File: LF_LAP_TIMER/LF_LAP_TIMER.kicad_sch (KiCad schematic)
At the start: 13 parts, among them J1 LCD I2C EXPANDER, K1 G6E, SW1 ARM, SW2 STOP, SW3 RESTART, SW4 OBJECT DETECTING

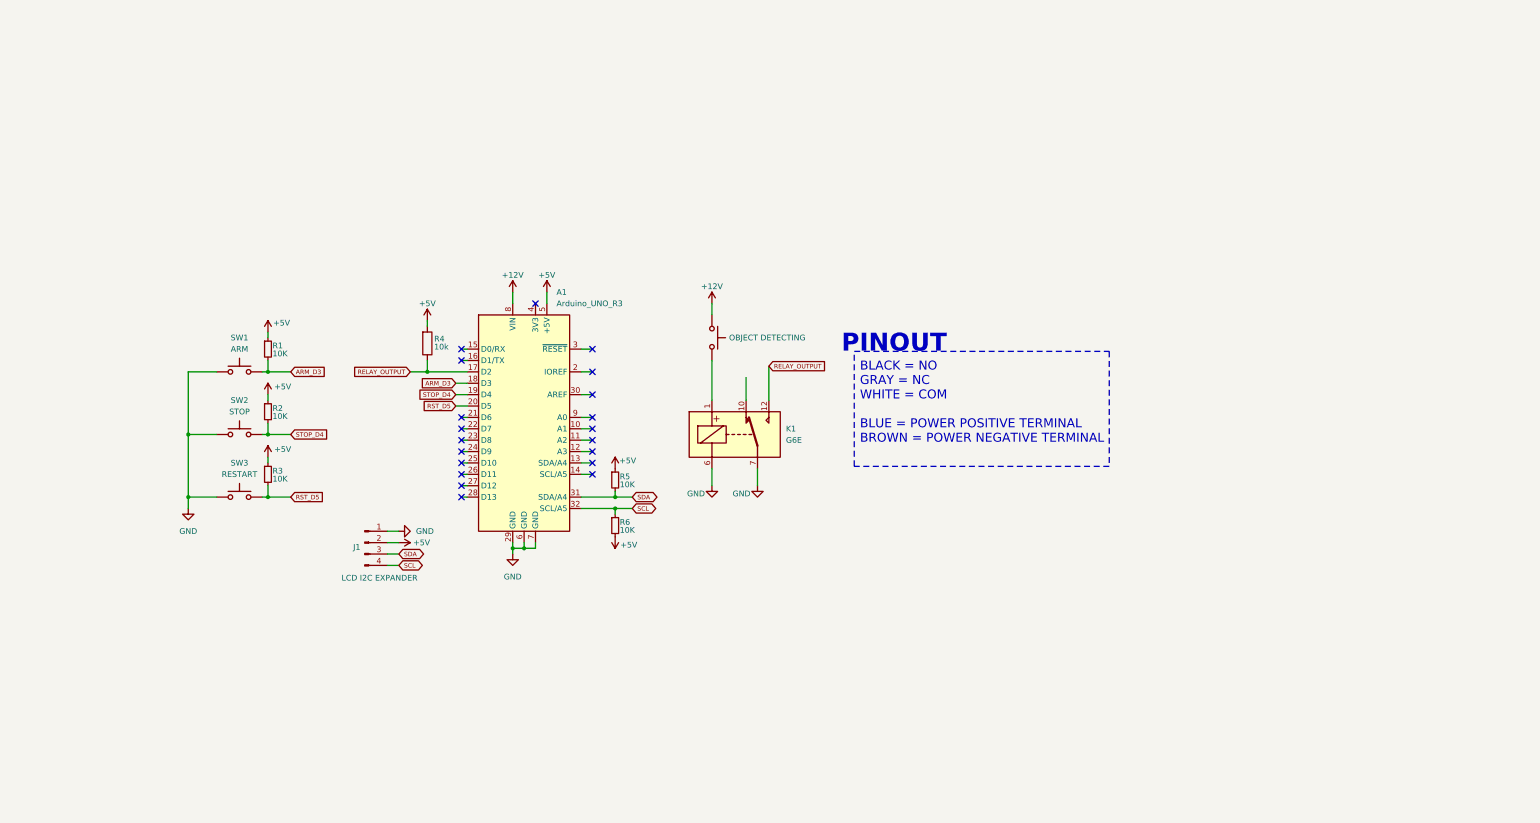
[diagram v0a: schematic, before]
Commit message: Footprint update
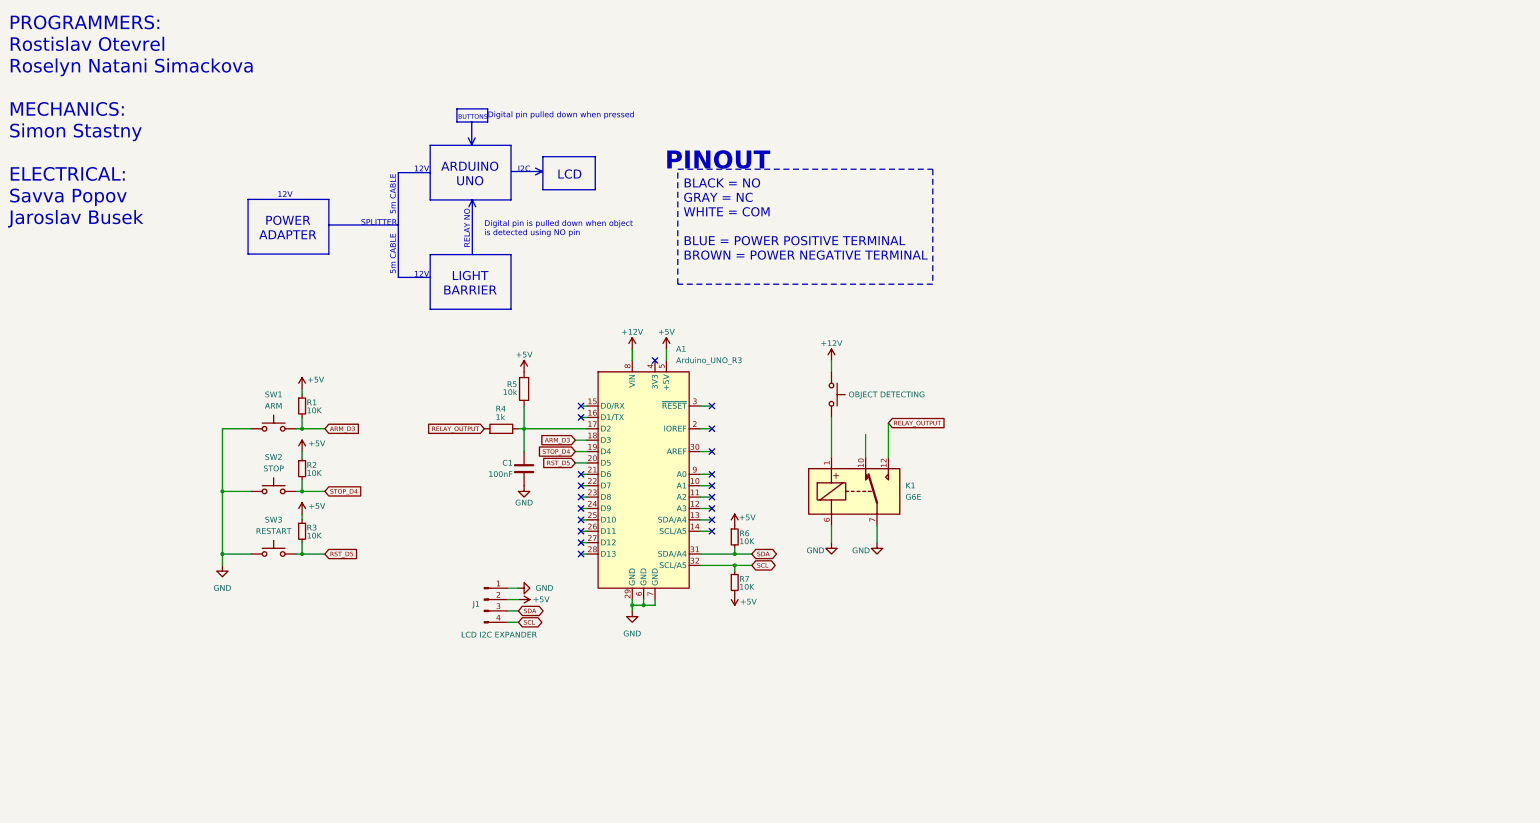
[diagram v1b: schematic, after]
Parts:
- added C1: 100nF, Capacitor_THT:C_Disc_D6.0mm_W2.5mm_P5.00mm, symbol Device:C
- added R4: 1k, Resistor_THT:R_Axial_DIN0207_L6.3mm_D2.5mm_P10.16mm_Horizontal, symbol Device:R
- J1: footprint (none) -> Connector_PinSocket_2.54mm:PinSocket_1x04_P2.54mm_Vertical
- K1: footprint Relay_THT:Relay_SPDT_Omron_G6E -> (none)
- R1, R2, R3: footprint (none) -> Resistor_THT:R_Axial_DIN0207_L6.3mm_D2.5mm_P10.16mm_Horizontal
- R5: renamed from R4; footprint (none) -> Resistor_THT:R_Axial_DIN0207_L6.3mm_D2.5mm_P10.16mm_Horizontal
- R6: renamed from R5; footprint (none) -> Resistor_THT:R_Axial_DIN0207_L6.3mm_D2.5mm_P10.16mm_Horizontal
- R7: renamed from R6; footprint (none) -> Resistor_THT:R_Axial_DIN0207_L6.3mm_D2.5mm_P10.16mm_Horizontal
- SW1, SW2, SW3: footprint (none) -> TerminalBlock:TerminalBlock_MaiXu_MX126-5.0-02P_1x02_P5.00mm
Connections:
- net GND: now also C1.2
- net RELAY_OUTPUT: now also R4.2; no longer A1.17 (D2), R5.1
- new net: A1.17 (D2), C1.1, R4.1, R5.1
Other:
- note added: "12V"
- note added: "5m CABLE"
- note added: "ARDUINO UNO"
- note added: "BUTTONS"
- note added: "Digital pin is pulled down when object is detected using NO pin"
- note added: "Digital pin pulled down when pressed"
- note added: "I2C"
- note added: "LCD"
- note added: "LIGHT BARRIER"
- note added: "POWER ADAPTER"
- note added: "PROGRAMMERS: Rostislav Otevrel Roselyn Natani Simackova MECHANICS: Simon Stastny ELECTRICAL: Savva Popov Jaroslav Busek"
- note added: "RELAY NO"
- note added: "SPLITTER"
- moved on the sheet: A1, J1, K1, R1, R2, R3, R5, R6, R7, SW1, SW2, SW3

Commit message: LF LAP TIMER
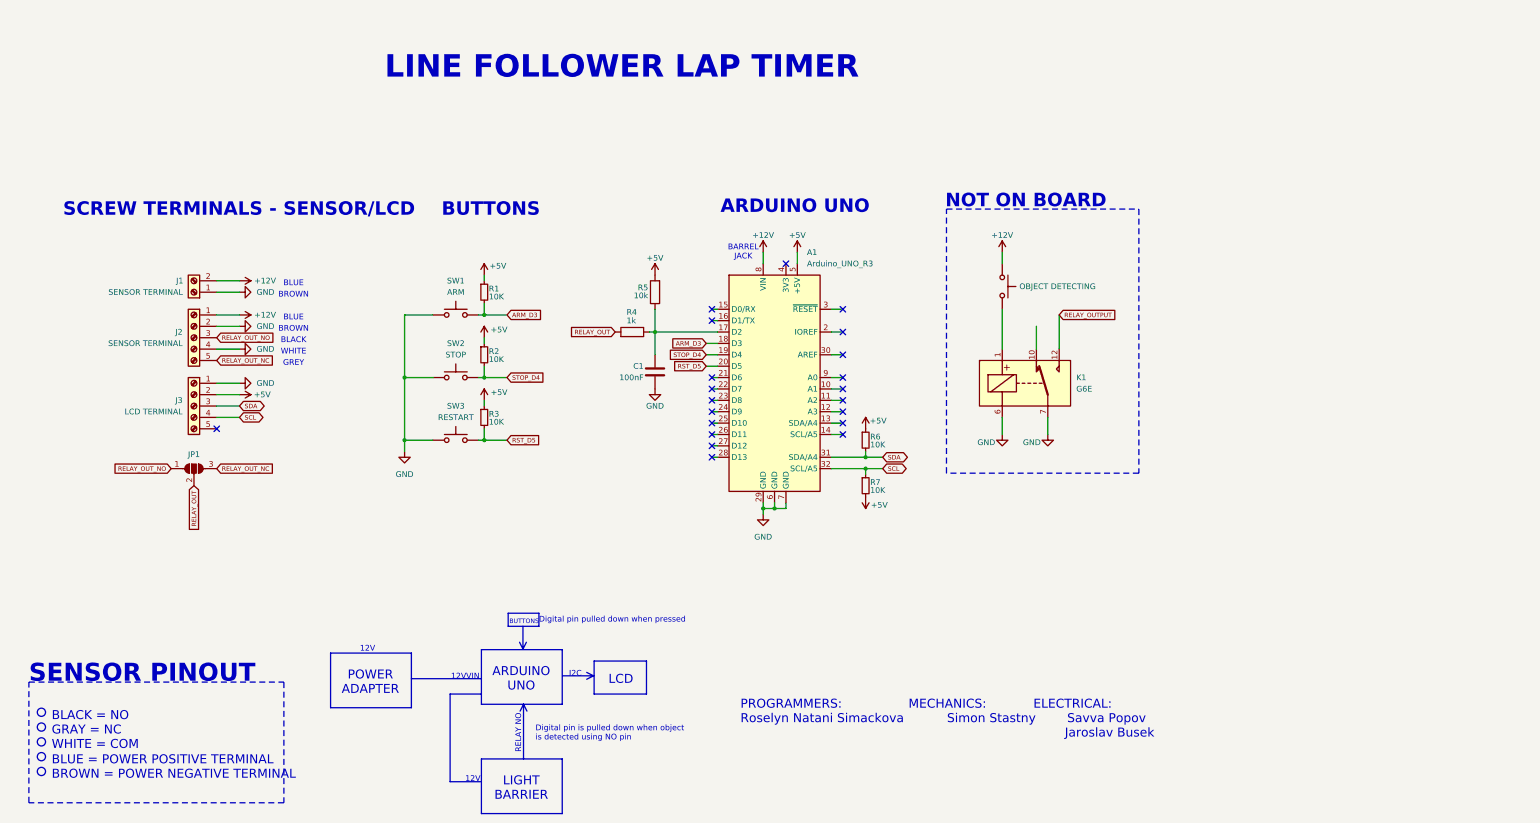
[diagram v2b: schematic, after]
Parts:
- removed J1: LCD I2C EXPANDER, Connector_PinSocket_2.54mm:PinSocket_1x04_P2.54mm_Vertical, symbol Connector:Conn_01x04_Pin
- added J1: SENSOR TERMINAL, TerminalBlock:TerminalBlock_MaiXu_MX126-5.0-02P_1x02_P5.00mm, symbol Connector:Screw_Terminal_01x02
- added J2: SENSOR TERMINAL, TerminalBlock:TerminalBlock_MaiXu_MX126-5.0-05P_1x05_P5.00mm, symbol Connector:Screw_Terminal_01x05
- added J3: LCD TERMINAL, TerminalBlock:TerminalBlock_MaiXu_MX126-5.0-05P_1x05_P5.00mm, symbol Connector:Screw_Terminal_01x05
- added JP1: SolderJumper_3_Open, Jumper:SolderJumper-3_P2.0mm_Open_TrianglePad1.0x1.5mm, symbol Jumper:SolderJumper_3_Open
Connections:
- net +12V: now also J1.2 (Pin_2), J2.1 (Pin_1)
- net +5V: now also J3.2 (Pin_2)
- net GND: now also J1.1 (Pin_1), J2.2 (Pin_2), J2.4 (Pin_4), J3.1 (Pin_1)
- net RELAY_OUTPUT: no longer R4.2
- net SCL: now also J3.4 (Pin_4)
- net SDA: now also J3.3 (Pin_3)
- new net RELAY_OUT: JP1.2 (C), R4.2
- new net RELAY_OUT_NC: J2.5 (Pin_5), JP1.3 (B)
- new net RELAY_OUT_NO: J2.3 (Pin_3), JP1.1 (A)
- no-connect marks 20 -> 21
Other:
- note added: "BARREL JACK"
- note added: "BLACK"
- note added: "BLACK = NO GRAY = NC WHITE = COM"
- note added: "BLUE"
- note added: "BLUE = POWER POSITIVE TERMINAL BROWN = POWER NEGATIVE TERMINAL"
- note added: "BROWN"
- note added: "GREY"
- note added: "LINE FOLLOWER LAP TIMER"
- note added: "NOT ON BOARD"
- note added: "PROGRAMMERS: MECHANICS: ELECTRICAL: Roselyn Natani Simackova Simon Stastny Savva Popov Jaroslav Busek"
- note added: "SCREW TERMINALS - SENSOR/LCD"
- note added: "SENSOR PINOUT"
- note added: "VIN"
- note added: "WHITE"
- note removed: "5m CABLE"
- note removed: "BLACK = NO GRAY = NC WHITE = COM BLUE = POWER POSITIVE TERMINAL BROWN = POWER NEGATIVE TERMINAL"
- note removed: "PINOUT"
- note removed: "PROGRAMMERS: Rostislav Otevrel Roselyn Natani Simackova MECHANICS: Simon Stastny ELECTRICAL: Savva Popov Jaroslav Busek"
- note removed: "SPLITTER"
- moved on the sheet: A1, C1, K1, R1, R2, R3, R4, R5, R6, R7, SW1, SW2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
